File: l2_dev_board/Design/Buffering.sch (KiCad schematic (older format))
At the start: 12 parts

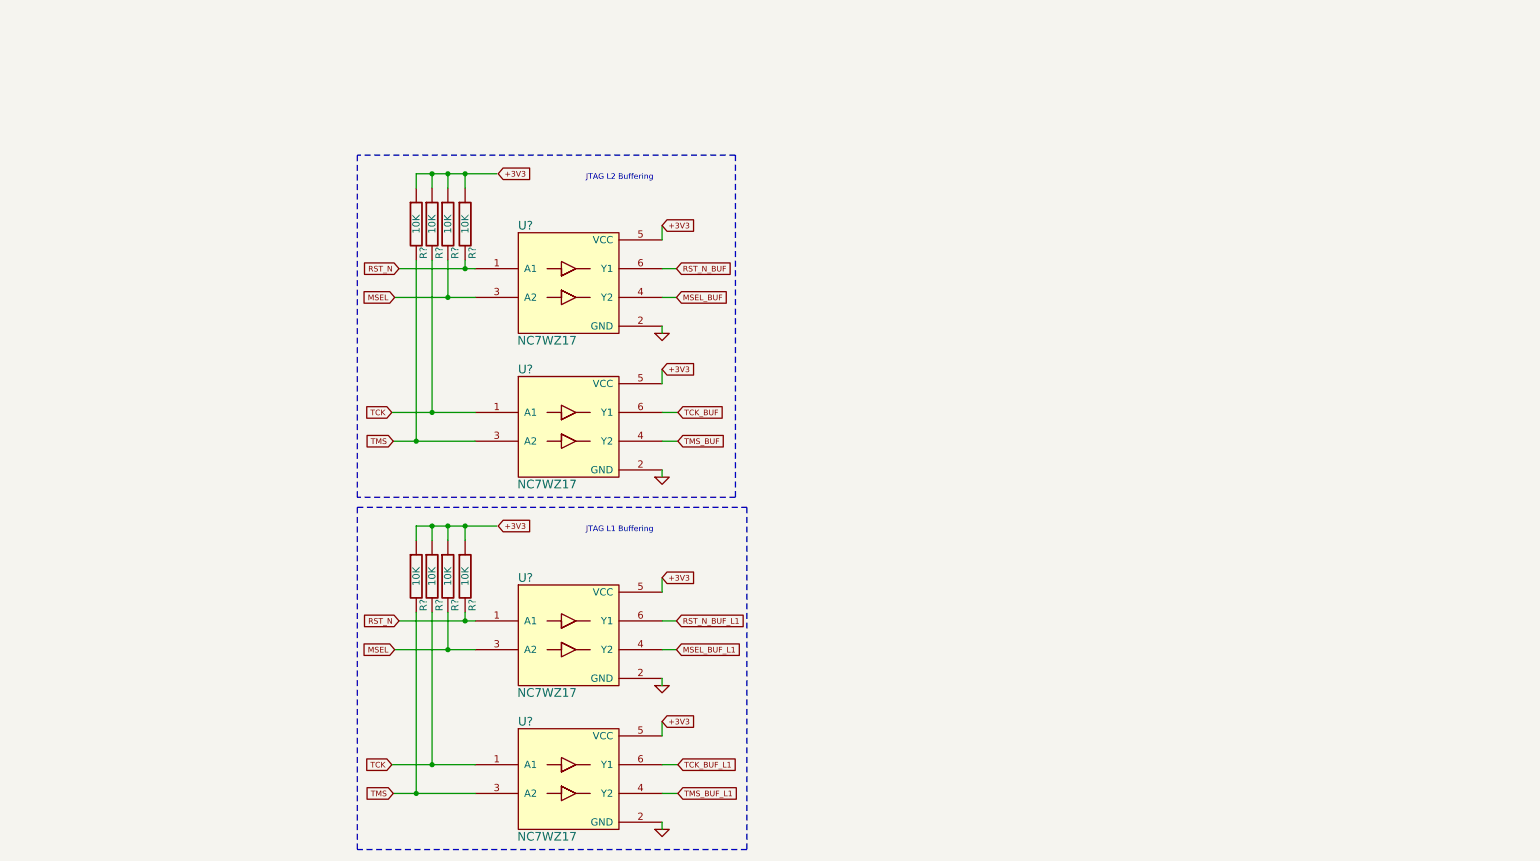
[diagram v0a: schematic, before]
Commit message: squash and back to work!
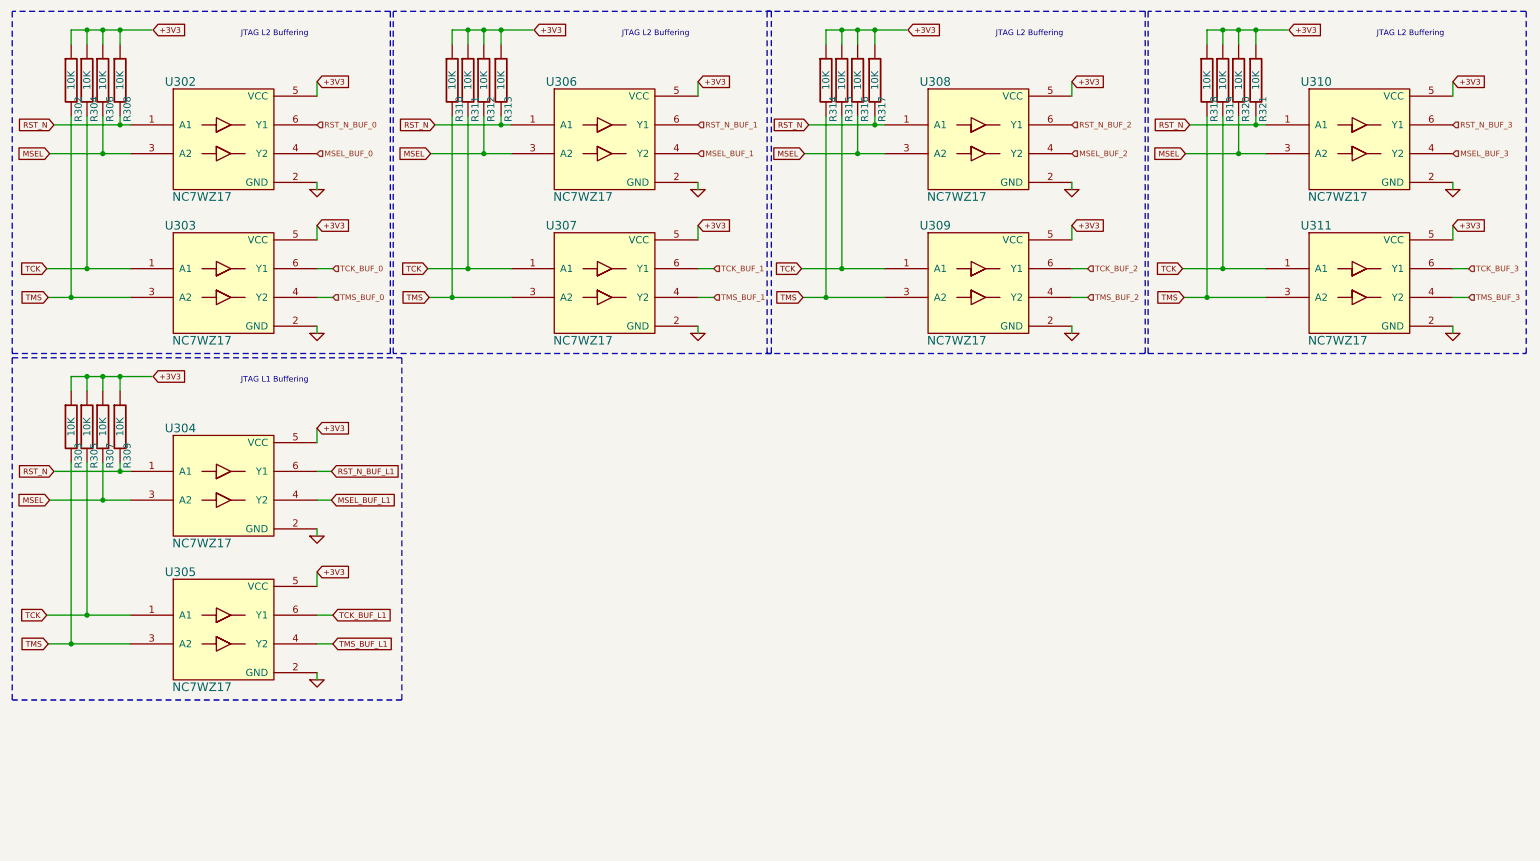
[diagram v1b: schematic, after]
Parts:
- added R310, R311, R312, R313, R314, R315, R316, R317, R318, R319, R320, R321: 10K, symbol R
- added U306, U307, U308, U309, U310, U311: NC7WZ17, symbol NC7WZ17
- gave numbers to parts that had none: 12
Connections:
- net labels added: MSEL_BUF_0, MSEL_BUF_1, MSEL_BUF_2, MSEL_BUF_3, RST_N_BUF_0, RST_N_BUF_1, RST_N_BUF_2, RST_N_BUF_3, TCK_BUF_0, TCK_BUF_1, TCK_BUF_2, TCK_BUF_3, TMS_BUF_0, TMS_BUF_1, TMS_BUF_2, TMS_BUF_3
- net labels removed: MSEL_BUF, RST_N_BUF, TCK_BUF, TMS_BUF
- wire segments 42 -> 104
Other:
- moved on the sheet: R302, R303, R304, R305, R306, R307, R308, R309, U302, U303, U304, U305
